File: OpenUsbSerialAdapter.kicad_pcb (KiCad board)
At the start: 2 copper layers, 39.8 x 16.4 mm, 21 parts, among them J1 USB_A, J2 FTDI, SW1 SW_DPDT_x2, U1 MCP2200-I-SO, U2 AMS1117-3.3, Y1 12M

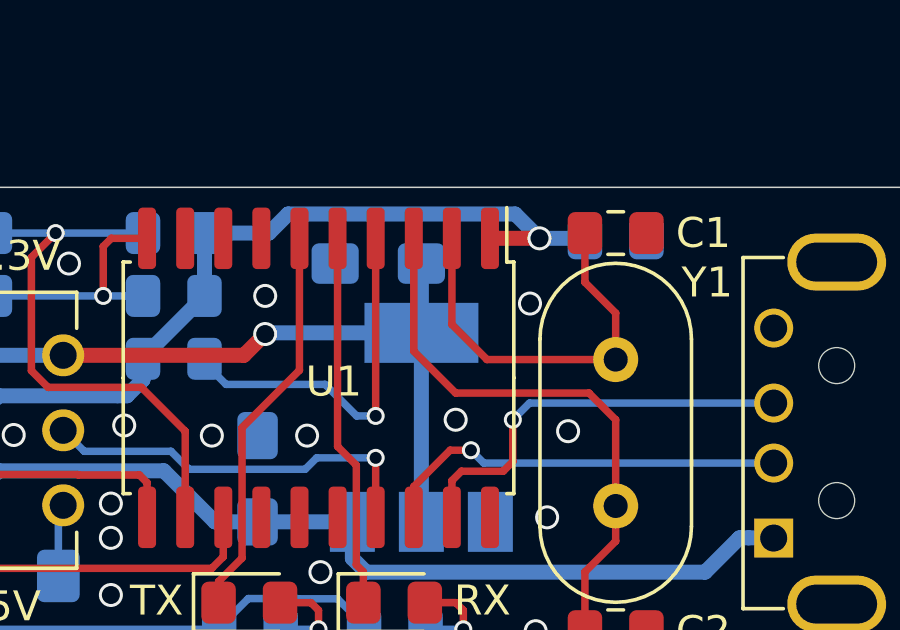
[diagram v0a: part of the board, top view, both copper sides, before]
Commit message: Tune quartz tracks length
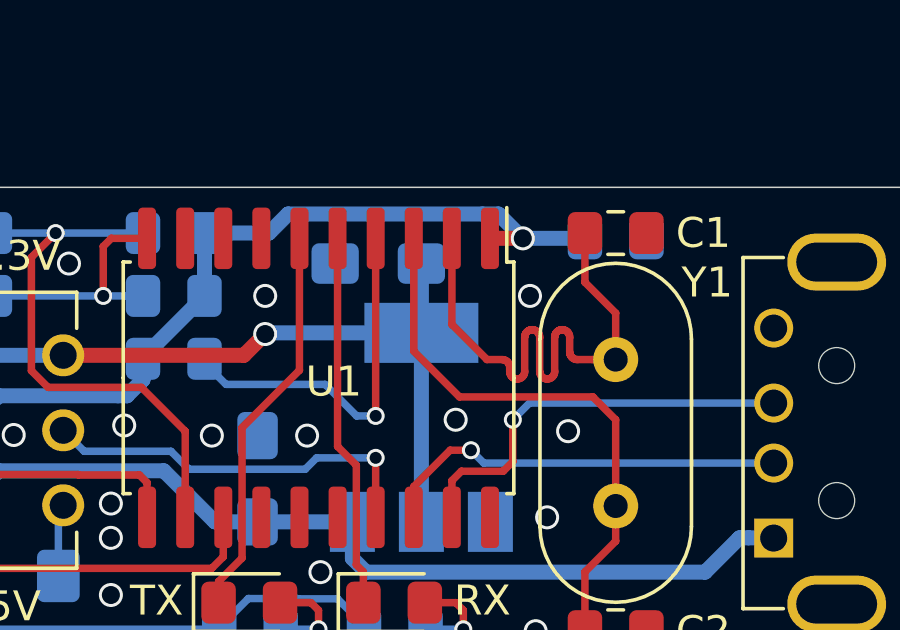
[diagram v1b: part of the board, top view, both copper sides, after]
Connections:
- net Net-(C1-Pad2) renamed /clk+
- net Net-(C2-Pad2) renamed /clk-
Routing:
- net /clk+: track 14.0 -> 19.5 mm
- net VCC: track 58.2 -> 57.7 mm
